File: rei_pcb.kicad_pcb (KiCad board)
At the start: 2 copper layers, 333.4 x 95.3 mm, 163 parts, among them J1 SM04B-SRSS-TB(LF)(SN), SW1 SW_Push, U2 ATmega32U4RC-MU, Y1 16MHz

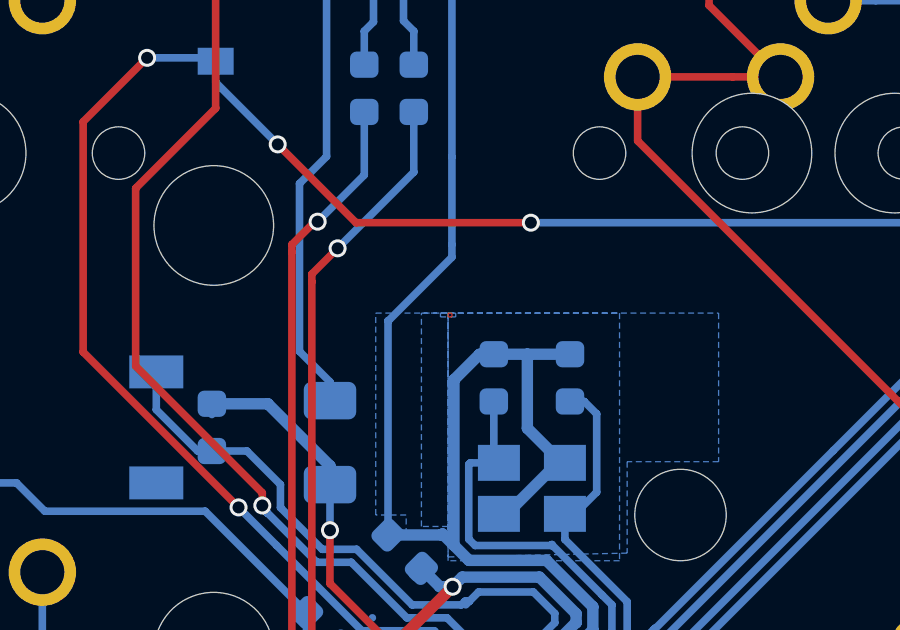
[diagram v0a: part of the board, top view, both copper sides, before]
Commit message: Gerber files
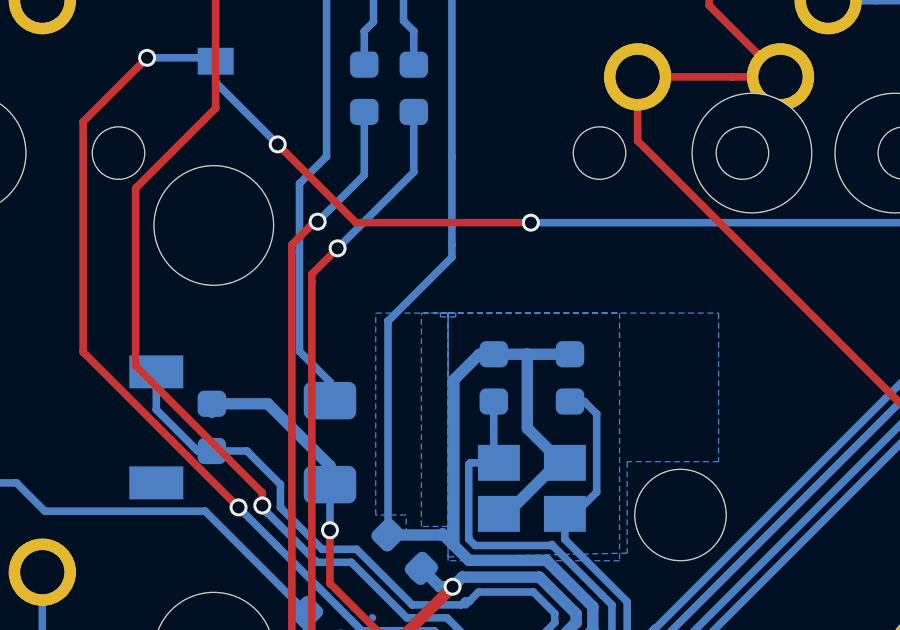
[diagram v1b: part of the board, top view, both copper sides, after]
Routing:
- removed copper zone on F.Cu, net GND
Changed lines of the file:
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@@
     (visible_elements 7FFFFFFF)
     (pcbplotparams
-      (layerselection 0x010fc_ffffffff)
-      (usegerberextensions false)
+      (layerselection 0x010f0_ffffffff)
+      (usegerberextensions true)
       (usegerberattributes false)
       (usegerberadvancedattributes false)
@@
       (outputformat 1)
       (mirror false)
-      (drillshape 1)
+      (drillshape 0)
       (scaleselection 1)
-      (outputdirectory ""))
+      (outputdirectory "Gerbers/"))
   )
   (net 0 "")
@@
       )
     )
-  )
-  (zone (net 1) (net_name GND) (layer F.Cu) (hatch edge 0.508)
-    (connect_pads (clearance 0.508))
-    (min_thickness 0.254)
-    (fill yes (arc_segments 32) (thermal_gap 0.508) (thermal_bridge_width 0.508))
-    (polygon
-      (pts
-        (xy 49.53 84.836) (xy 49.403 84.836) (xy 49.403 84.709) (xy 49.53 84.709)
-      )
-    )
